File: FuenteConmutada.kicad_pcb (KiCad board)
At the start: 2 copper layers, 9 parts, among them J2 Conn_01x02_Socket, P1 USB_C_Plug_USB2.0, U1 MT3608

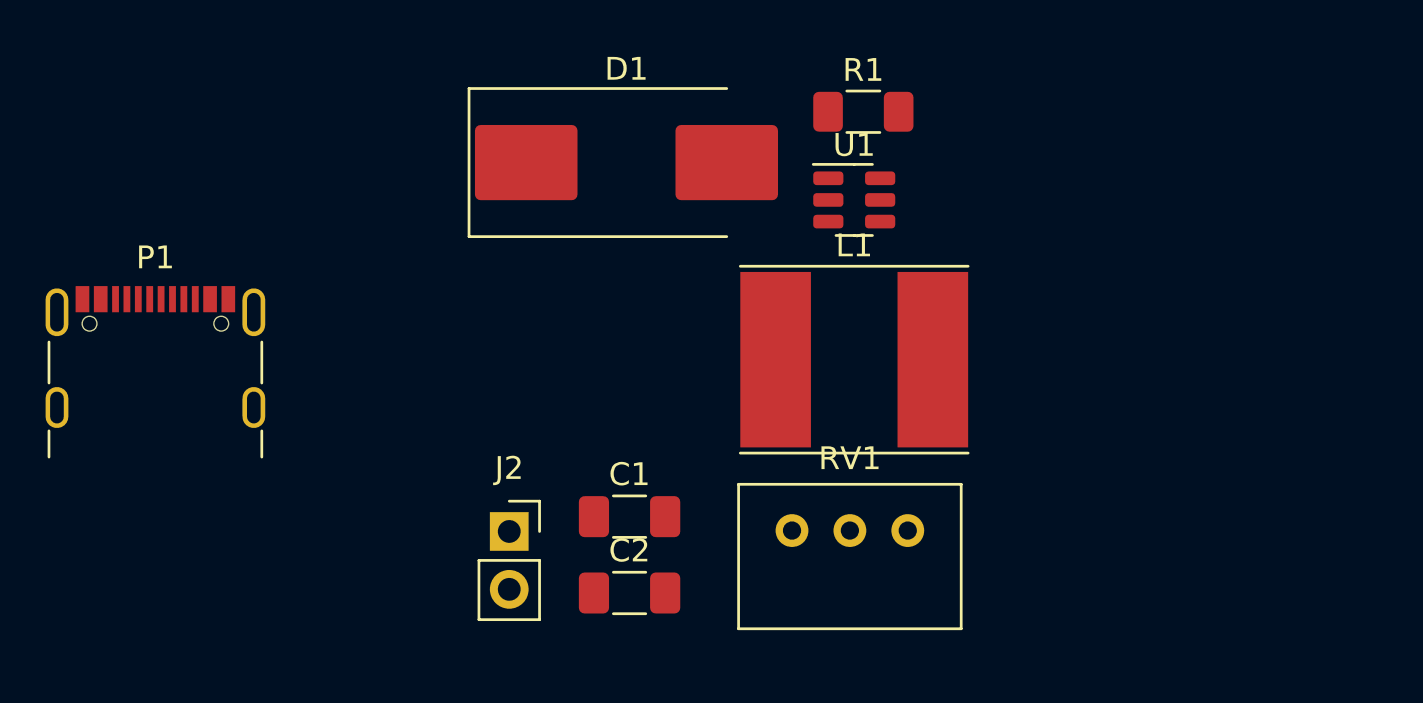
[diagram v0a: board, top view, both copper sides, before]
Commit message: avance en ruteo
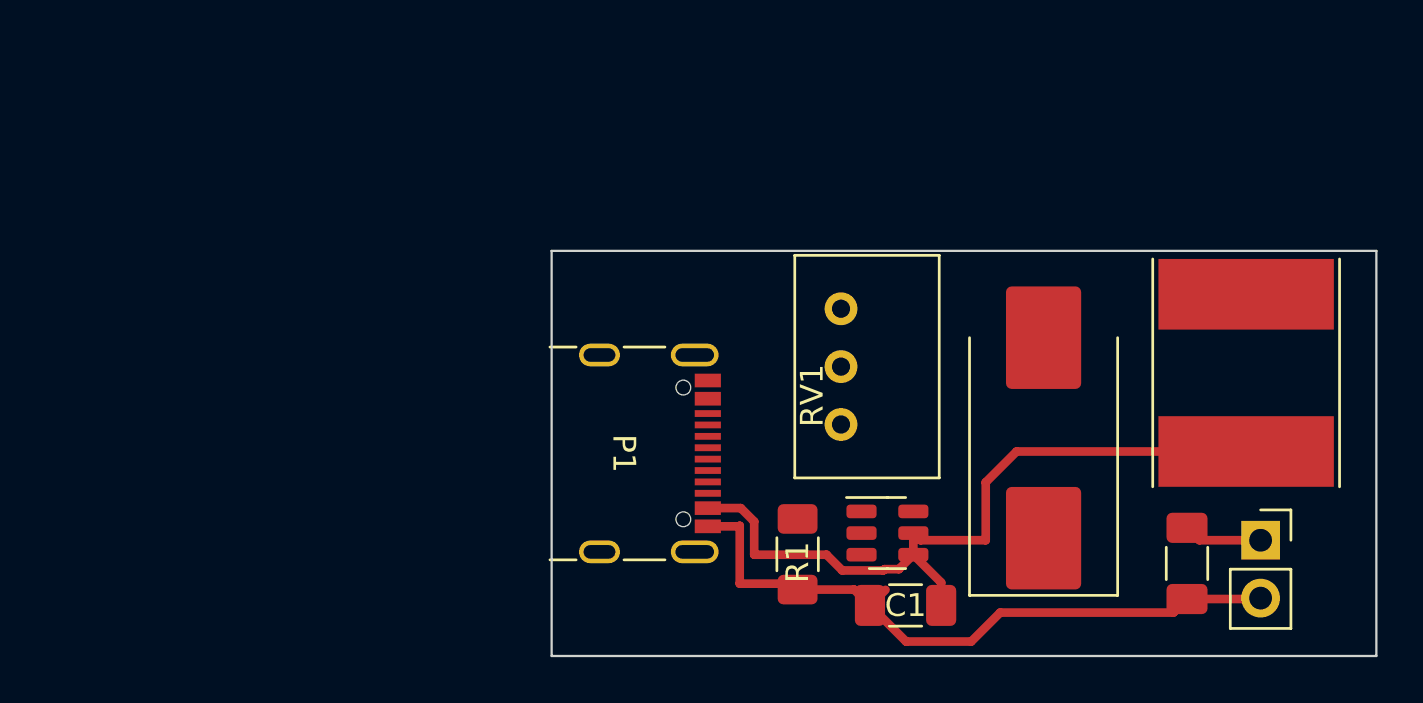
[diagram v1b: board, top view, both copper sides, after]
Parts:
- moved J2 33.0 mm to (108.6, 73.0)
- moved C2 24.5 mm to (105.4, 74.0), turned to 90 degrees
- moved D1 21.9 mm to (99.1, 68.5), turned to 90 degrees
- moved P1 20.8 mm to (80.6, 69.2), turned to -90 degrees
- moved R1 19.6 mm to (88.3, 73.6), turned to -90 degrees
- moved L1 17.2 mm to (108.0, 65.7), turned to 90 degrees
- moved U1 14.7 mm to (92.2, 72.7)
- moved C1 12.7 mm to (93.0, 75.9)
- moved RV1 10.2 mm to (90.2, 62.9), turned to 90 degrees
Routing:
- net Net-(U1-EN): track 0.00 -> 33.3 mm
- net GND: track 0.00 -> 29.6 mm
- net Net-(J2-Pin_1): track 0.00 -> 3.46 mm
- net Net-(U1-SW): track 0.00 -> 1.04 mm
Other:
- board outline added: 36.2 x 17.8 mm
